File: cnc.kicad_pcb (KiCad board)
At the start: 2 copper layers, 99.1 x 99.1 mm, 62 parts, among them J1 Micro_SD_Card_Det, J10 Conn_01x04_Male, J11 Conn_01x04_Male, J12 Conn_01x02_Male, J13 Conn_01x02_Male, J14 Conn_01x02_Male, J15 Conn_01x02_Male, J16 Screw_Terminal_01x02, J2 Conn_01x02_Male, J3 Conn_01x02_Male, J4 Conn_01x04_Male, J5 Conn_01x04_Male, J6 Conn_01x02_Male, J7 Conn_01x02_Male, J8 Conn_01x02_Male, J9 Conn_01x02_Male, U1 LM324, U2 ESP32-DEVKITC, U3 AOZ1282CI, U4 AZ1117-3.3

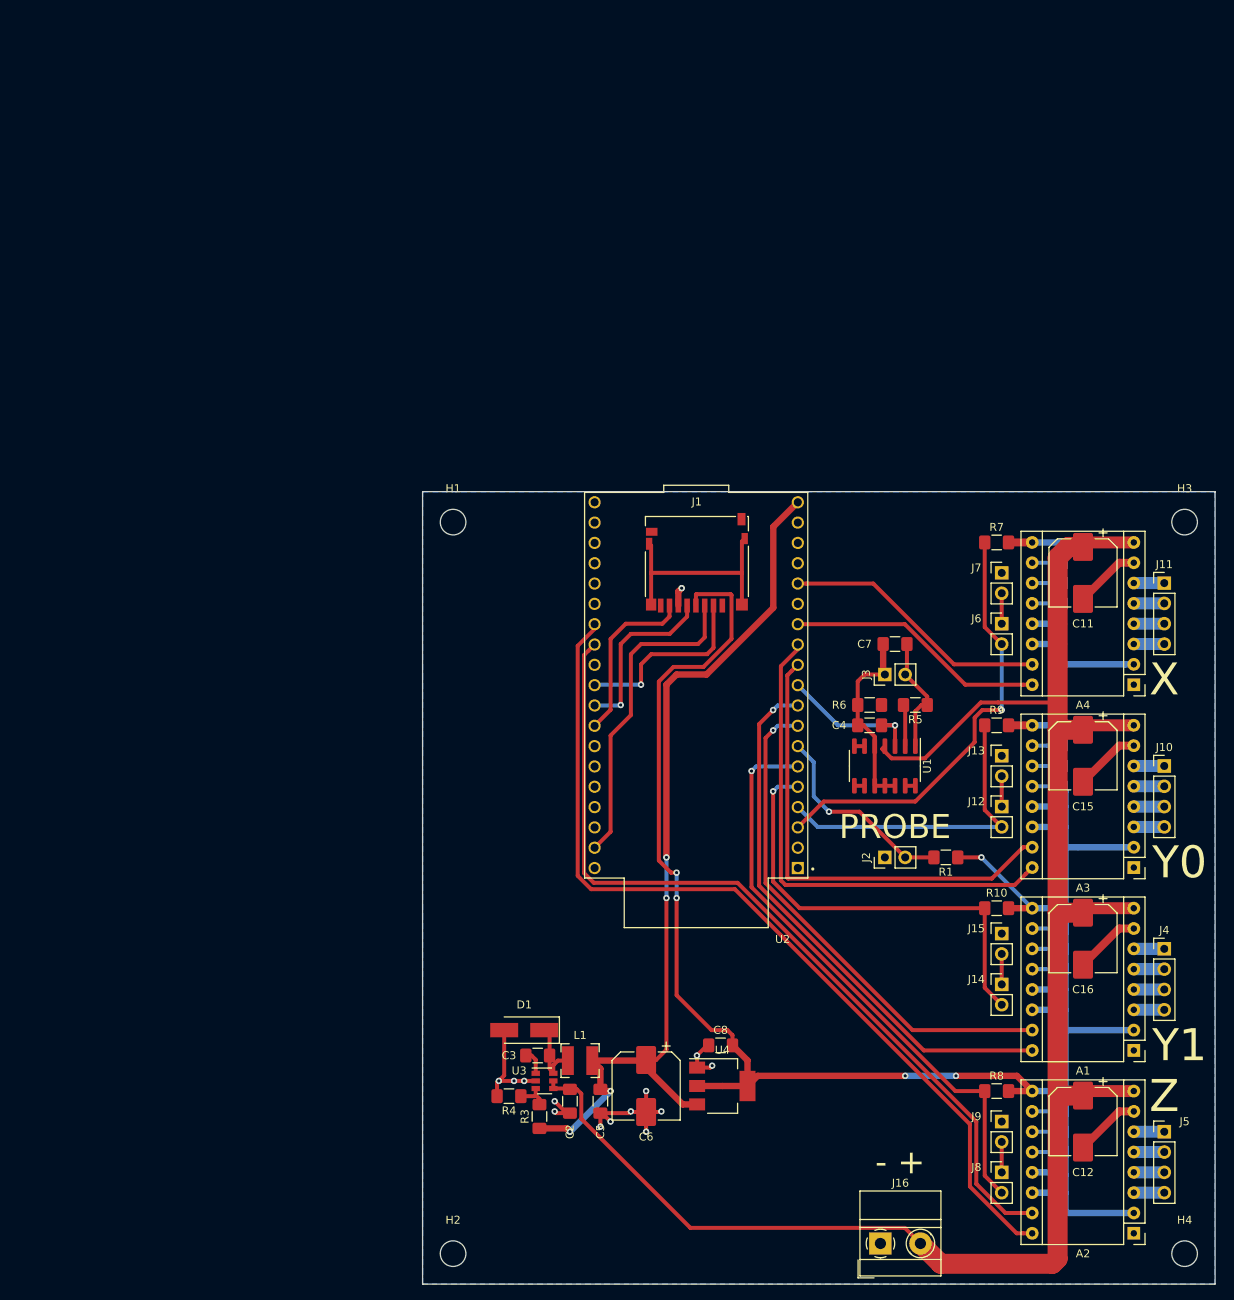
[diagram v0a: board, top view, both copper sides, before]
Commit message: Fixes
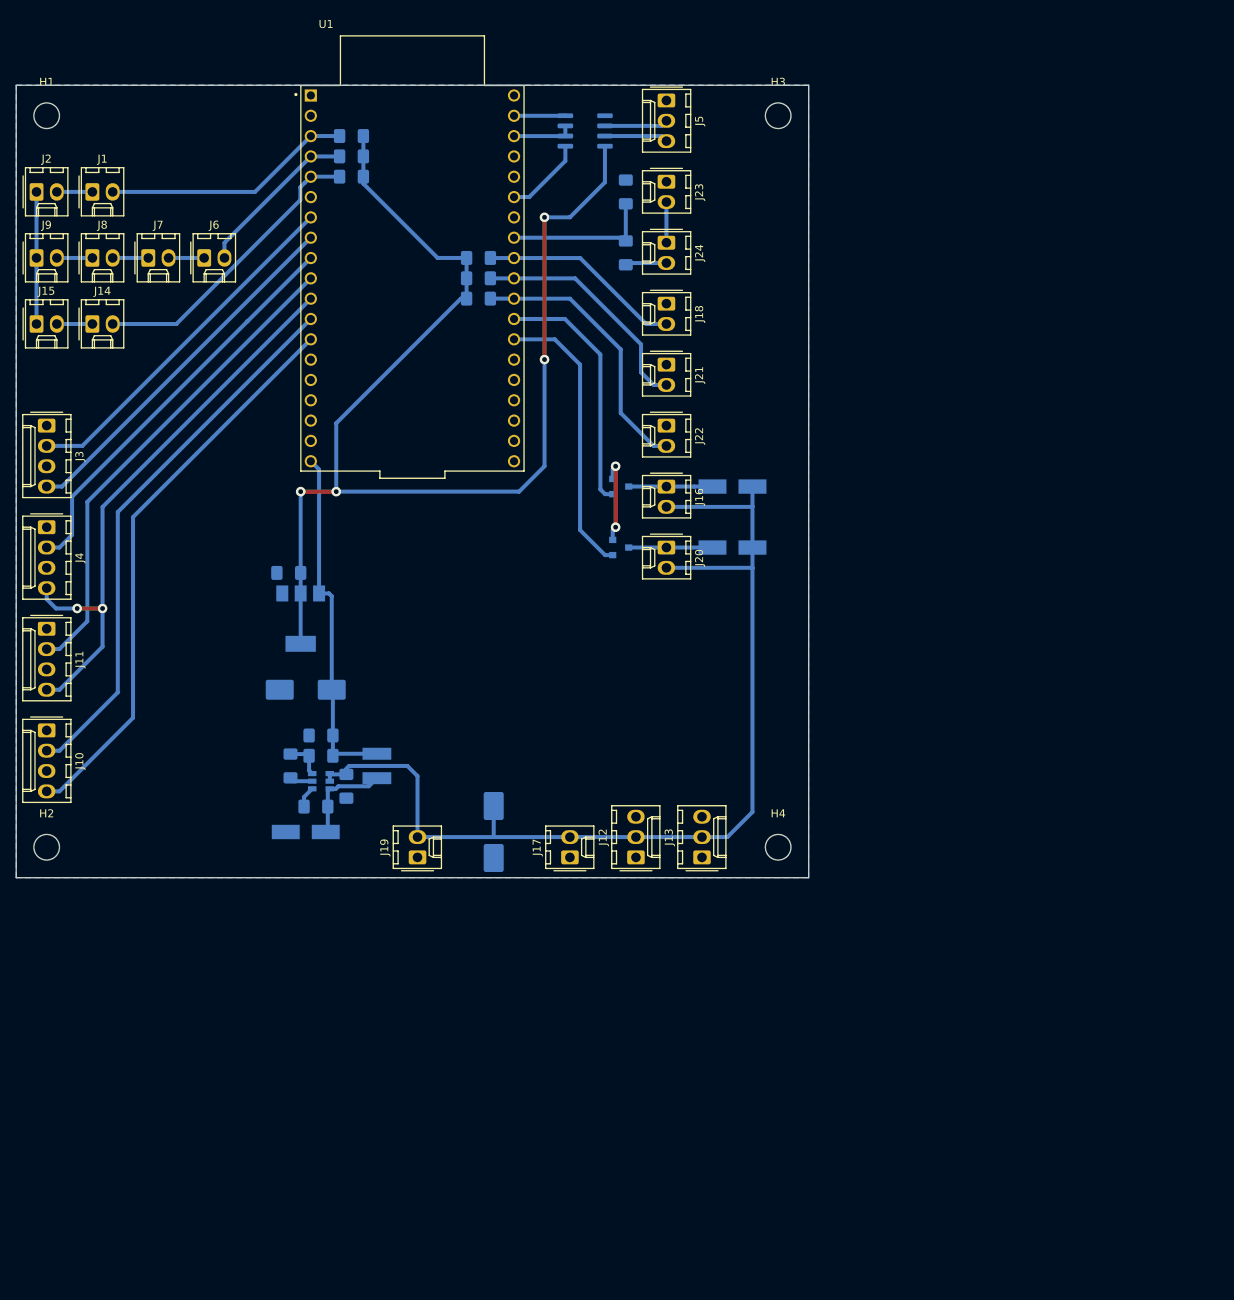
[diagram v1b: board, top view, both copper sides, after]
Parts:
- removed A1, A2, A3, A4: Pololu_Breakout_A4988, Module:Pololu_Breakout-16_15.2x20.3mm
- removed C11, C12, C15, C16: 100u, Capacitor_SMD:CP_Elec_8x10
- removed C7: 100n, Capacitor_SMD:C_1206_3216Metric_Pad1.42x1.75mm_HandSolder
- removed C8: 10u, Capacitor_SMD:C_1206_3216Metric_Pad1.42x1.75mm_HandSolder
- removed JP1, JP10, JP11, JP12, JP2, JP3, JP4, JP5, JP6, JP7, JP8, JP9: SolderJumper_2_Open, Jumper:SolderJumper-2_P1.3mm_Open_Pad1.0x1.5mm
- added C1: 470u, Capacitor_SMD:CP_Elec_8x10, B.Cu at (59.7, 93.3)
- added D2: D_Schottky, Diode_SMD:D_SMA_Handsoldering, B.Cu at (89.5, 50.2)
- added D3: D_Schottky, Diode_SMD:D_SMA_Handsoldering, B.Cu at (89.5, 57.8)
- added J17: Conn_01x02_Male, Connector_Molex:Molex_KK-254_AE-6410-02A_1x02_P2.54mm_Vertical, F.Cu at (69.2, 96.5)
- added J18: Conn_01x02_Male, Connector_Molex:Molex_KK-254_AE-6410-02A_1x02_P2.54mm_Vertical, F.Cu at (81.3, 27.3)
- added J19: Conn_01x02_Male, Connector_Molex:Molex_KK-254_AE-6410-02A_1x02_P2.54mm_Vertical, F.Cu at (50.2, 96.5)
- added J20: Conn_01x02_Male, Connector_Molex:Molex_KK-254_AE-6410-02A_1x02_P2.54mm_Vertical, F.Cu at (81.3, 57.8)
- added J21: Conn_01x02_Male, Connector_Molex:Molex_KK-254_AE-6410-02A_1x02_P2.54mm_Vertical, F.Cu at (81.3, 34.9)
- added J22: Conn_01x02_Male, Connector_Molex:Molex_KK-254_AE-6410-02A_1x02_P2.54mm_Vertical, F.Cu at (81.3, 42.5)
- added J23: Conn_01x02_Male, Connector_Molex:Molex_KK-254_AE-6410-02A_1x02_P2.54mm_Vertical, F.Cu at (81.3, 12.1)
- added J24: Conn_01x02_Male, Connector_Molex:Molex_KK-254_AE-6410-02A_1x02_P2.54mm_Vertical, F.Cu at (81.3, 19.7)
- added Q1: DMG2302U, Package_TO_SOT_SMD:SOT-23, B.Cu at (75.6, 50.2)
- added Q2: DMG2302U, Package_TO_SOT_SMD:SOT-23, B.Cu at (75.6, 57.8)
- added R2: 1k, Resistor_SMD:R_1206_3216Metric_Pad1.42x1.75mm_HandSolder, B.Cu at (34.3, 85.1)
- C2, C3, D1, L1, R10, R4, R7, R9: moved to B.Cu
- C4: value 100n -> 10u; moved to B.Cu
- C5: value 10u -> 470u; footprint Capacitor_SMD:C_1206_3216Metric_Pad1.42x1.75mm_HandSolder -> Capacitor_SMD:CP_Elec_8x10; moved to B.Cu
- C6: value 470u -> 10u; footprint Capacitor_SMD:CP_Elec_8x10 -> Capacitor_SMD:C_1206_3216Metric_Pad1.42x1.75mm_HandSolder; moved to B.Cu
- J1: value Micro_SD_Card_Det -> Conn_01x02_Male; footprint Connector_Card:microSD_HC_Hirose_DM3D-SF -> Connector_Molex:Molex_KK-254_AE-6410-02A_1x02_P2.54mm_Vertical
- J10, J11, J4: footprint Connector_PinHeader_2.54mm:PinHeader_1x04_P2.54mm_Vertical -> Connector_Molex:Molex_KK-254_AE-6410-04A_1x04_P2.54mm_Vertical
- J12, J13: value Conn_01x02_Male -> Conn_01x03_Male; footprint Connector_PinHeader_2.54mm:PinHeader_1x02_P2.54mm_Vertical -> Connector_Molex:Molex_KK-254_AE-6410-03A_1x03_P2.54mm_Vertical
- J14, J15, J2, J6, J7, J8, J9: footprint Connector_PinHeader_2.54mm:PinHeader_1x02_P2.54mm_Vertical -> Connector_Molex:Molex_KK-254_AE-6410-02A_1x02_P2.54mm_Vertical
- J16: value Screw_Terminal_01x02 -> Conn_01x02_Male; footprint TerminalBlock_MetzConnect:TerminalBlock_MetzConnect_Type011_RT05502HBWC_1x02_P5.00mm_Horizontal -> Connector_Molex:Molex_KK-254_AE-6410-02A_1x02_P2.54mm_Vertical
- J3: value Conn_01x02_Male -> Conn_01x04_Male; footprint Connector_PinHeader_2.54mm:PinHeader_1x02_P2.54mm_Vertical -> Connector_Molex:Molex_KK-254_AE-6410-04A_1x04_P2.54mm_Vertical
- J5: value Conn_01x04_Male -> Conn_01x03_Male; footprint Connector_PinHeader_2.54mm:PinHeader_1x04_P2.54mm_Vertical -> Connector_Molex:Molex_KK-254_AE-6410-03A_1x03_P2.54mm_Vertical
- R1: value 1k -> 4k7; moved to B.Cu
- R3: value 4k7 -> 1k; moved to B.Cu
- R5: value 33k -> 1k; moved to B.Cu
- R6: value 10k -> 1k; moved to B.Cu
- R8: value 1k -> 6k8; moved to B.Cu
- U1: value LM324 -> ESP32-DEVKITC; footprint Package_SO:SOIC-14_3.9x8.7mm_P1.27mm -> parts:MODULE_ESP32-DEVKITC
- U2: value ESP32-DEVKITC -> AOZ1282CI; footprint parts:MODULE_ESP32-DEVKITC -> Package_TO_SOT_SMD:SOT-23-6; moved to B.Cu
- U3: value AOZ1282CI -> AZ1117-3.3; footprint Package_TO_SOT_SMD:SOT-23-6 -> Package_TO_SOT_SMD:SOT-223-3_TabPin2; moved to B.Cu
- U4: value AZ1117-3.3 -> ST485EBDR; footprint Package_TO_SOT_SMD:SOT-223-3_TabPin2 -> Package_SO:SOIC-8_3.9x4.9mm_P1.27mm; moved to B.Cu
- moved J9 161.9 mm to (2.54, 21.6)
- moved J8 161.2 mm to (9.53, 21.6)
- moved J4 149.3 mm to (3.81, 55.2), turned to 270 degrees
- moved J5 143.1 mm to (81.3, 1.91), turned to 270 degrees
- moved J15 142.7 mm to (2.54, 29.8)
- moved J14 140.5 mm to (9.53, 29.8)
- moved J11 139.8 mm to (3.81, 67.9), turned to 270 degrees
- moved J10 139.8 mm to (3.81, 80.6), turned to 270 degrees
- moved J2 134.8 mm to (2.54, 13.3), turned to 0 degrees
- moved R3 124.8 mm to (41.9, 6.35), turned to 180 degrees
- moved U4 120.6 mm to (71.1, 5.71)
- moved R4 119.1 mm to (41.9, 8.89)
- moved R8 114.6 mm to (76.2, 21.0), turned to 90 degrees
- moved J7 113.7 mm to (16.5, 21.6)
- moved J6 109.7 mm to (23.5, 21.6)
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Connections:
- C2 pad 1: +24V -> +12V
- C4 pad 1: SPINDLE -> +5V
- C6 pad 1: +5V -> +3V3
- J1 pad 1: (no net) -> Net-(J1-Pad1)
- J1 pad 2: CS -> LIMIT_X
- J10 pad 1: Net-(A3-Pad6) -> GND
- J10 pad 2: Net-(A3-Pad5) -> STEP_Z
- J10 pad 3: Net-(A3-Pad4) -> GND
- J10 pad 4: Net-(A3-Pad3) -> DIR_Z
- J11 pad 1: Net-(A4-Pad6) -> GND
- J11 pad 2: Net-(A4-Pad5) -> STEP_Y1
- J11 pad 3: Net-(A4-Pad4) -> GND
- J11 pad 4: Net-(A4-Pad3) -> DIR_Y
- J12 pad 1: Net-(J12-Pad1) -> GND
- J12 pad 2: LIMIT_Y0 -> +12V
- J13 pad 2: Net-(J12-Pad1) -> +12V
- J14 pad 2: LIMIT_Y1 -> LIMIT_Z
- J16 pad 1: GND -> Net-(D2-Pad2)
- J16 pad 2: +24V -> +12V
- J2 pad 2: PROBE -> Net-(J1-Pad1)
- J3 pad 2: Net-(C7-Pad1) -> STEP_X
- J4 pad 1: Net-(A1-Pad6) -> GND
- J4 pad 2: Net-(A1-Pad5) -> STEP_Y0
- J4 pad 3: Net-(A1-Pad4) -> GND
- J4 pad 4: Net-(A1-Pad3) -> DIR_Y
- J5 pad 1: Net-(A2-Pad6) -> GND
- J5 pad 2: Net-(A2-Pad5) -> Net-(J5-Pad2)
- J5 pad 3: Net-(A2-Pad4) -> Net-(J5-Pad3)
- J6 pad 2: LIMIT_X -> LIMIT_Y
- J7 pad 1: GND -> Net-(J7-Pad1)
- J8 pad 2: LIMIT_Z -> Net-(J7-Pad1)
- R1 pad 1: +3V3 -> +5V
- R1 pad 2: PROBE -> Net-(R1-Pad2)
- R10 pad 2: LIMIT_Y1 -> CYCLE_START
- R3 pad 1: +5V -> +3V3
- R3 pad 2: Net-(R3-Pad2) -> LIMIT_X
- R4 pad 1: Net-(R3-Pad2) -> +3V3
- R4 pad 2: GND -> LIMIT_Y
- R5 pad 1: Net-(C7-Pad1) -> +3V3
- R5 pad 2: Net-(R5-Pad2) -> LIMIT_Z
- R6 pad 1: Net-(R5-Pad2) -> +3V3
- R6 pad 2: GND -> PROBE
- R7 pad 2: LIMIT_X -> FEED_HOLD
- R8 pad 1: +3V3 -> Net-(J24-Pad2)
- R8 pad 2: LIMIT_Z -> E_STOP
- R9 pad 1: +3V3 -> E_STOP
- R9 pad 2: LIMIT_Y0 -> GND
- U1 pad 1: Net-(C7-Pad1) -> (no net)
- U1 pad 10: GND -> STEP_Y1
- U1 pad 11: GND -> DIR_Y
- U1 pad 12: GND -> STEP_Z
- U1 pad 13: Net-(U1-Pad13) -> DIR_Z
- U1 pad 14: Net-(U1-Pad13) -> GND
- U1 pad 2: Net-(R5-Pad2) -> (no net)
- U1 pad 3: SPINDLE -> LIMIT_X
- U1 pad 4: +24V -> LIMIT_Y
- U1 pad 5: GND -> LIMIT_Z
- U1 pad 6: Net-(U1-Pad6) -> (no net)
- U1 pad 7: Net-(U1-Pad6) -> STEP_X
- U1 pad 8: Net-(U1-Pad8) -> DIR_X
- U1 pad 9: Net-(U1-Pad8) -> STEP_Y0
- U2 pad 1: (no net) -> Net-(C3-Pad1)
- U2 pad 2: (no net) -> GND
- U2 pad 3: LIMIT_X -> Net-(R1-Pad2)
- U2 pad 4: LIMIT_Y0 -> +12V
- U2 pad 5: LIMIT_Y1 -> +12V
- U2 pad 6: LIMIT_Z -> Net-(C3-Pad2)
- U3 pad 1: Net-(C3-Pad1) -> GND
- U3 pad 2: GND -> +3V3
- U3 pad 3: Net-(R3-Pad2) -> +5V
- U4 pad 1: GND -> RX
- U4 pad 2: +3V3 -> RTS
- U4 pad 3: +5V -> RTS
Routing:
- net +24V: track 228.0 -> 0.00 mm
- net +3V3: track 313.7 -> 154.9 mm, vias 5 -> 4
- net +12V: track 0.00 -> 130.2 mm
- net DIR_Y: track 0.00 -> 72.3 mm, vias 0 -> 2
- net GND: track 99.3 -> 30.5 mm, vias 14 -> 2
- net +5V: track 113.0 -> 44.3 mm, vias 4 -> 0
- net DIR_Y0: track 62.9 -> 0.00 mm
- net LIMIT_Y1: track 55.4 -> 0.00 mm, vias 1 -> 0
- net DIR_Z: track 112.2 -> 71.1 mm
- net MOSI: track 40.1 -> 0.00 mm
- net LIMIT_Y0: track 40.1 -> 0.00 mm
- net STEP_Z: track 107.3 -> 68.6 mm
- net LIMIT_Z: track 73.8 -> 36.9 mm, vias 1 -> 0
- net COOLANT: track 0.00 -> 35.6 mm
- net CYCLE_START: track 0.00 -> 34.3 mm
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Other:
- board text removed: "- +"
- board text removed: "PROBE"
- board text removed: "X"
- board text removed: "Y0"
- board text removed: "Y1"
- board text removed: "Z"
